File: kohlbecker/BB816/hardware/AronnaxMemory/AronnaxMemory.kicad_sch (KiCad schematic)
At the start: 29 parts, among them J1 Barrel_Jack_Switch, J2 Conn_02x40_Odd_Even, J3 Conn_02x18_Odd_Even, J5 I/O ~{CS}, J9 Vector Rewrite, U1 74LS04, U12 AS6C4008-55PCN, U13 AT28C256-15PC, U2 74LS32, U3 74LS32, U4 74LS08, U6 74LS32, U7 74LS32, U8 74LS138

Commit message: Cleanup
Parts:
- removed C6, C8: 100nF, Capacitor_THT:C_Disc_D3.4mm_W2.1mm_P2.50mm, symbol Device:C
- removed unit 4 of U2
- removed unit 5 of U2
- removed unit 2 of U2
- removed unit 1 of U2
- removed unit 1 of U6
- removed U7: 74LS32, Package_DIP:DIP-14_W7.62mm, symbol 74xx:74LS32
- removed U8: 74LS138, Package_DIP:DIP-16_W7.62mm, symbol 74xx:74LS138
- added C10, C11: 100nF, Capacitor_THT:C_Disc_D3.4mm_W2.1mm_P2.50mm, symbol Device:C
- added U10: 74HC30, Package_DIP:DIP-14_W7.62mm, symbol BB816:74HC30
- added U9: CD4072B, Package_DIP:DIP-14_W7.62mm, symbol cd4072B:4072
- renumbered U2 to U6
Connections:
- net A10: now also U10.2; no longer U6.5
- net A11: now also U10.3
- net A12: now also U10.4
- net A13: now also U10.5
- net A14: now also U10.6
- net A15: now also U1.1, U3.13; no longer U1.5, U3.10
- net A19: now also U1.9, U6.2; no longer U1.11, U6.10
- net A20: now also U9.5
- net A21: now also U9.4
- net A22: now also U9.3
- net A23: now also U9.2
- net A8: now also U10.11
- net A9: now also U10.12; no longer U6.4
- net E: now also U1.11, U4.13; no longer U1.1, U4.5
- net GND: now also J9.15 (Pin_15), J9.17 (Pin_17), J9.19 (Pin_19), J9.21 (Pin_21), U1.5, U4.4, U4.5, U6.10, U6.4, U6.5, U6.9, C10.2, C11.2, U10.7 (GND), U9.10, U9.11, U9.12, U9.7 (VSS), U9.9; no longer U1.9, U4.12, U4.13
- net VCC: now also C10.1, C11.1, U10.14 (VCC), U9.14 (VDD)
- net ~{BANK0_HI}: now also U1.13; no longer U1.3
- net ~{BANK0_LO}: now also U3.11, U10.1; no longer U3.8
- net ~{BANK0}: now also U3.12; no longer U3.9
- net ~{MEG0_LO}: now also U6.3; no longer U6.8
- net ~{PAGE1}: now also U1.4; no longer U1.13
- net ~{ROM_OE}: no longer U13.22 (~{OE})
- net at U3.4: now also U1.10; no longer U1.2
- net at U6.6: no longer U6.9
- net ~{A19}: now reaches U1.8
- net ~{A19}: now also U6.12
- net at U4.11: now also U3.9
- net ~{MEG0}: now reaches U6.13
- net ~{MEG0}: now also U6.1, U9.1; no longer U6.9
- net ~{MEG0_LO_OE}: now reaches U12.24 (OE#)
- net ~{MEG0_LO_OE}: now also U3.8; no longer U3.11
- net at U4.6: no longer U3.12
- net at U1.12: now also U4.12; no longer U3.13
- net at U1.6: no longer U3.1
- net ~{0x00}: no longer names the net of J5.20 (Pin_20)
- net ~{0x20}: no longer names the net of J5.18 (Pin_18)
- net ~{0x40}: no longer names the net of J5.16 (Pin_16)
- net ~{0x60}: no longer names the net of J5.14 (Pin_14)
- net ~{0x80}: no longer names the net of J5.12 (Pin_12)
- net ~{0xA0}: no longer names the net of J5.10 (Pin_10)
- net ~{0xCO}: no longer names the net of J5.8 (Pin_8)
- net ~{0xE0}: no longer names the net of J5.6 (Pin_6)
- new net PAGE1: U1.3, U10.8, U3.10
- new net ~{A15}: U1.2, U3.1
- no-connect marks 5 -> 8
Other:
- removed sheet VectorPullRewrite
- moved on the sheet: C1, C12, C13, C2, C3, C4, C5, C7, C9, D1, H1, H2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

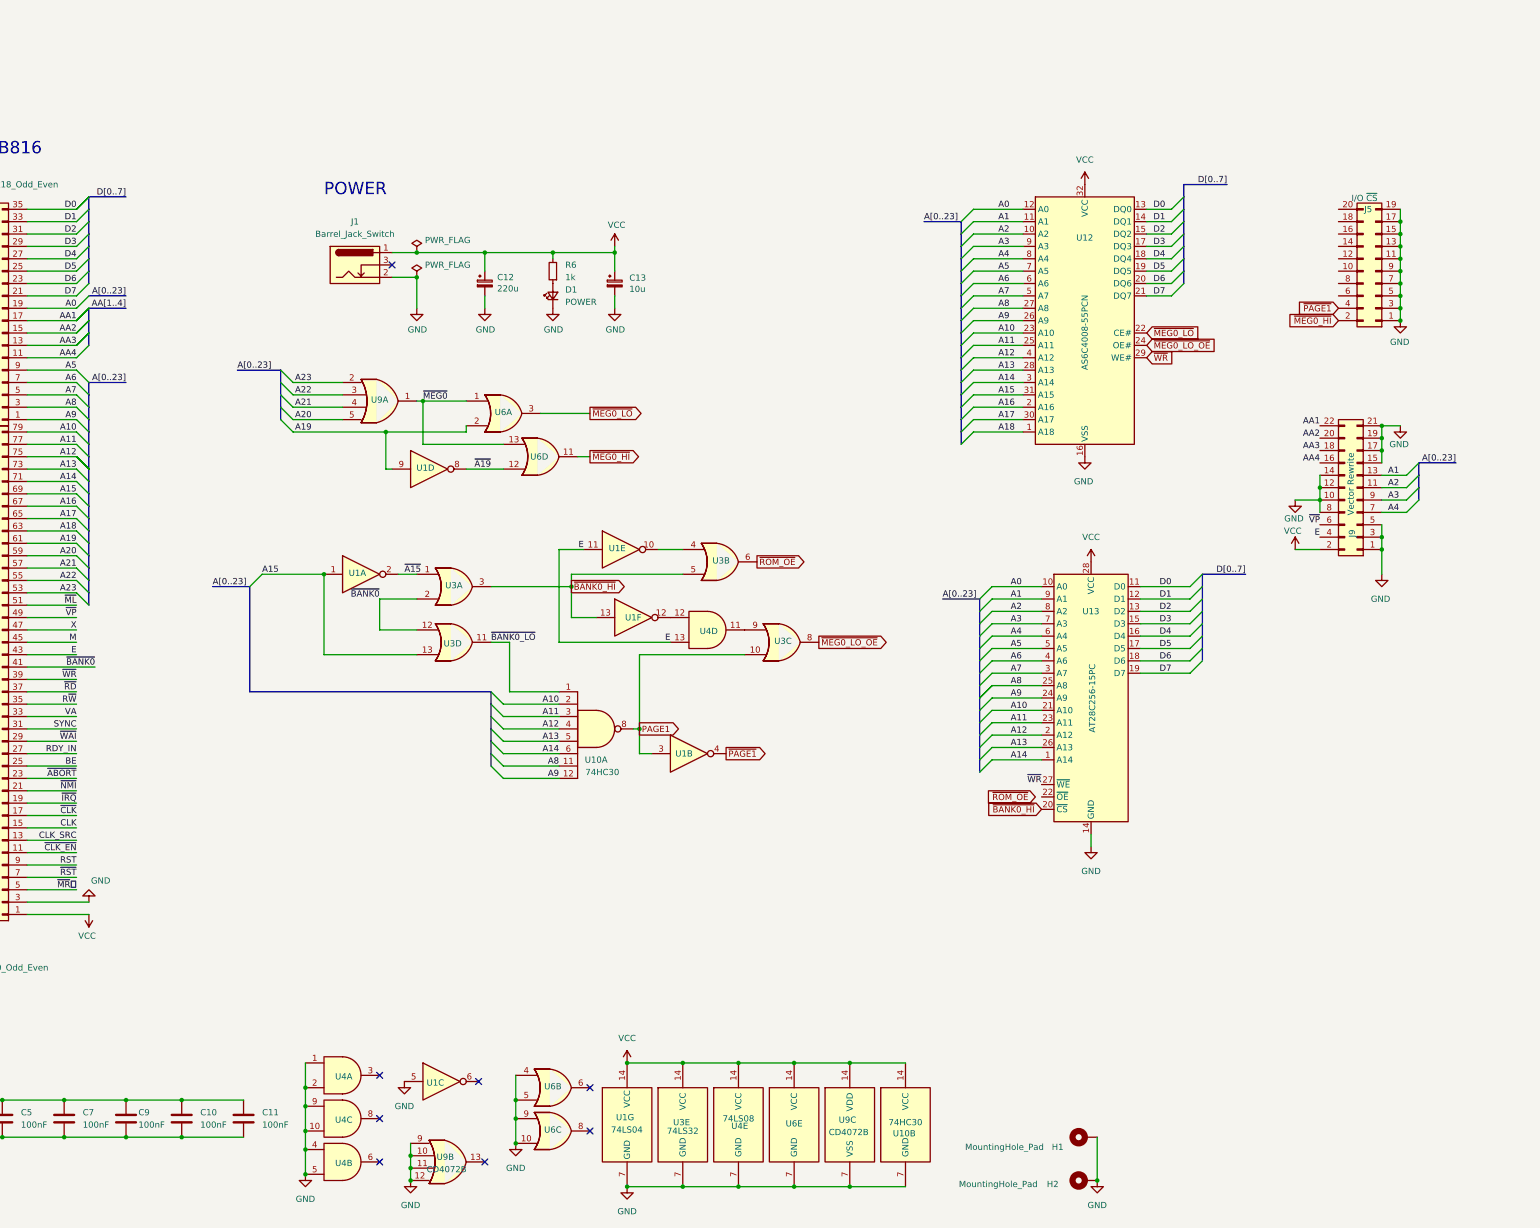
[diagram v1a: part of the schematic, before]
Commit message: ATF22V10
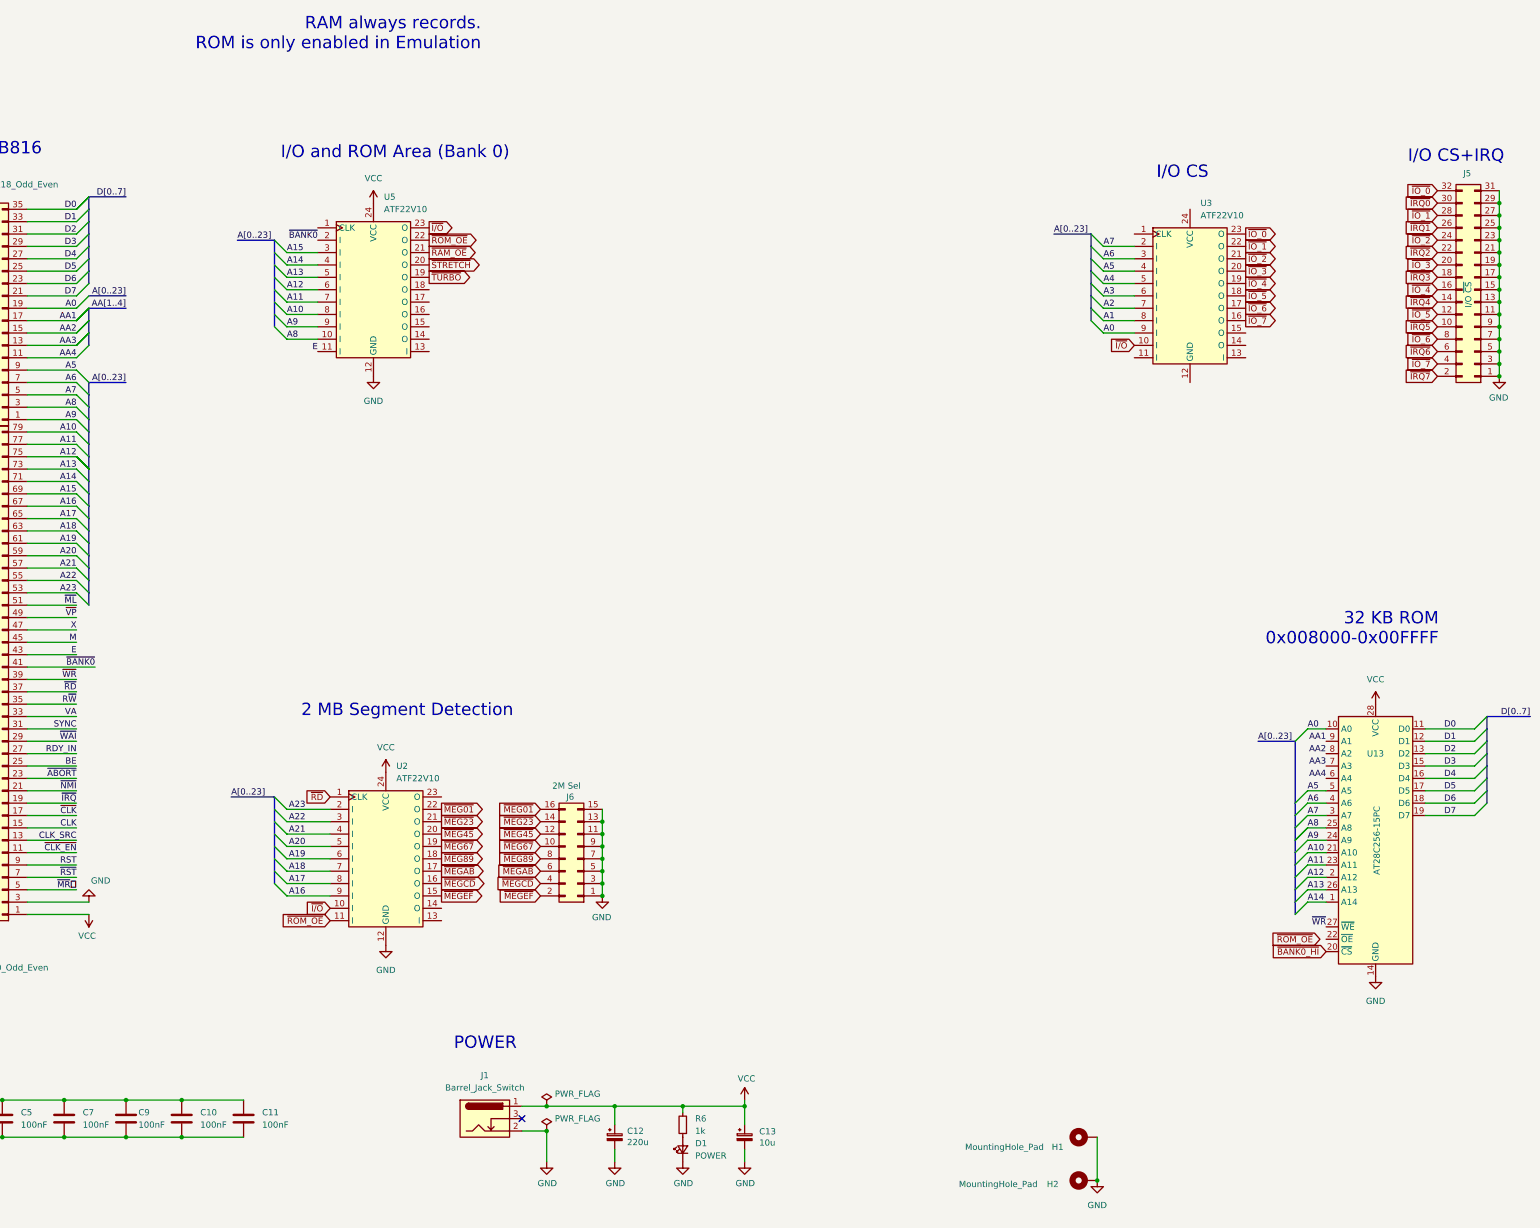
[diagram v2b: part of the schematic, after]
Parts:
- removed J9: Vector Rewrite, Connector_PinHeader_2.54mm:PinHeader_2x11_P2.54mm_Vertical, symbol Connector_Generic:Conn_02x11_Odd_Even
- removed U1: 74LS04, Package_DIP:DIP-14_W7.62mm, symbol 74xx:74LS04
- removed U10: 74HC30, Package_DIP:DIP-14_W7.62mm, symbol BB816:74HC30
- removed U12: AS6C4008-55PCN, Package_DIP:DIP-32_W15.24mm, symbol Memory_RAM:AS6C4008-55PCN
- removed U3, U6: 74LS32, Package_DIP:DIP-14_W7.62mm, symbol 74xx:74LS32
- removed U4: 74LS08, Package_DIP:DIP-14_W7.62mm, symbol 74xx:74LS08
- removed U9: CD4072B, Package_DIP:DIP-14_W7.62mm, symbol cd4072B:4072
- added J6: 2M Sel, Connector_PinHeader_2.54mm:PinHeader_2x10_P2.54mm_Vertical, symbol Connector_Generic:Conn_02x08_Odd_Even
- added U2, U3, U5: ATF22V10, Package_DIP:DIP-24_W7.62mm_Socket, symbol my:ATF22V10
- J5: symbol Connector_Generic:Conn_02x10_Odd_Even -> Connector_Generic:Conn_02x16_Odd_Even
- U13: footprint Socket:DIP_Socket-28_W11.9_W12.7_W15.24_W17.78_W18.5_3M_228-1277-00-0602J -> Package_DIP:DIP-28_W15.24mm_Socket
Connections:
- net A0: now also U3.9 (I)
- net A1: now also U3.8 (I); no longer U13.9 (A1)
- net A10: now also U5.8 (I)
- net A11: now also U5.7 (I)
- net A12: now also U5.6 (I)
- net A13: now also U5.5 (I)
- net A14: now also U5.4 (I)
- net A15: now also U5.3 (I)
- net A16: now also U2.9 (I)
- net A17: now also U2.8 (I)
- net A18: now also U2.7 (I)
- net A19: now also U2.6 (I)
- net A2: now also U3.7 (I); no longer U13.8 (A2)
- net A20: now also U2.5 (I)
- net A21: now also U2.4 (I)
- net A22: now also U2.3 (I)
- net A23: now also U2.2 (I)
- net A3: now also U3.6 (I); no longer U13.7 (A3)
- net A4: now also U3.5 (I); no longer U13.6 (A4)
- net A5: now also U3.4 (I)
- net A6: now also U3.3 (I)
- net A7: now also U3.2 (I)
- net A8: now also U5.10 (I)
- net A9: now also U5.9 (I)
- net AA1: now also U13.9 (A1)
- net AA2: now also U13.8 (A2)
- net AA3: now also U13.7 (A3)
- net AA4: now also U13.6 (A4)
- net E: now also U5.11 (I)
- net GND: now also J5.21 (Pin_21), J5.23 (Pin_23), J5.25 (Pin_25), J5.27 (Pin_27), J5.29 (Pin_29), J5.31 (Pin_31), J6.1 (Pin_1), J6.11 (Pin_11), J6.13 (Pin_13), J6.15 (Pin_15), J6.3 (Pin_3), J6.5 (Pin_5), J6.7 (Pin_7), J6.9 (Pin_9), U2.12 (GND), U5.12 (GND)
- net VCC: now also U2.24 (VCC), U5.24 (VCC)
- net ~{BANK0}: now also U5.2 (I)
- net ~{RD}: now also U2.1 (CLK)
- net ~{ROM_OE}: now also U2.11 (I), U5.22 (O)
- net ~{IRQ5}: now reaches J5.10 (Pin_10)
- net ~{IO_5}: now reaches J5.12 (Pin_12)
- net ~{IO_5}: now also U3.18 (O)
- net ~{IRQ4}: now reaches J5.14 (Pin_14)
- net ~{IO_4}: now reaches J5.16 (Pin_16)
- net ~{IO_4}: now also U3.19 (O)
- net ~{IRQ3}: now reaches J5.18 (Pin_18)
- net ~{IO_3}: now reaches J5.20 (Pin_20)
- net ~{IO_3}: now also U3.20 (O)
- net ~{IRQ6}: now reaches J5.6 (Pin_6)
- net ~{IO_6}: now reaches J5.8 (Pin_8)
- net ~{IO_6}: now also U3.17 (O)
- net ~{MEG0_HI} renamed ~{IRQ7}
- net ~{PAGE1} renamed ~{IO_7}
- net ~{IO_7}: now also U3.16 (O)
- new net ~{IO_0}: J5.32 (Pin_32), U3.23 (O)
- new net ~{IO_1}: J5.28 (Pin_28), U3.22 (O)
- new net ~{IO_2}: J5.24 (Pin_24), U3.21 (O)
- new net ~{IRQ0}: J5.30 (Pin_30)
- new net ~{IRQ1}: J5.26 (Pin_26)
- new net ~{IRQ2}: J5.22 (Pin_22)
- new net ~{I/O}: U2.10 (I), U3.10 (I), U5.23 (O)
- new net ~{MEG01}: J6.16 (Pin_16), U2.22 (O)
- new net ~{MEG23}: J6.14 (Pin_14), U2.21 (O)
- new net ~{MEG45}: J6.12 (Pin_12), U2.20 (O)
- new net ~{MEG67}: J6.10 (Pin_10), U2.19 (O)
- new net ~{MEG89}: J6.8 (Pin_8), U2.18 (O)
- new net ~{MEGAB}: J6.6 (Pin_6), U2.17 (O)
- new net ~{MEGCD}: J6.4 (Pin_4), U2.16 (O)
- new net ~{MEGEF}: J6.2 (Pin_2), U2.15 (O)
- new net ~{RAM_OE}: U5.21 (O)
- new net ~{STRETCH}: U5.20 (O)
- new net ~{TURBO}: U5.19 (O)
- no-connect marks 8 -> 1
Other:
- note added: "2 MB Segment Detection"
- note added: "32 KB ROM 0x008000-0x00FFFF"
- note added: "I/O CS"
- note added: "I/O CS+IRQ"
- note added: "I/O and ROM Area (Bank 0)"
- note added: "RAM always records. ROM is only enabled in Emulation"
- moved on the sheet: C12, C13, D1, J1, R6, U13

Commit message: PLAs for Days! Also Vector Rewrite
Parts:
- added D2, D3: 1N4148, Diode_THT:D_DO-35_SOD27_P7.62mm_Horizontal, symbol Diode:1N4148
- added J7: ~{IRQ7_NMI}, symbol Connector_Generic:Conn_02x02_Odd_Even
- added R1, R15: 1K, symbol Device:R
- added R13, R14, R3, R4, R5: 10K, symbol Device:R
- added RN1: 100k, Resistor_THT:R_Array_SIP9, symbol Device:R_Network08
- added U4: 74HC283, Package_DIP:DIP-16_W7.62mm_Socket, symbol Vega816:74HC283
- added U89: 74LS348, Package_DIP:DIP-16_W7.62mm_Socket, symbol 74xx:74LS348
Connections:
- net A1: now also U4.5 (A1)
- net A2: now also U4.3 (A2)
- net A3: now also U4.14 (A3)
- net A4: now also U4.12 (A4)
- net AA1: now also U4.10 (S4)
- net AA2: now also U4.13 (S3)
- net AA3: now also U4.1 (S2)
- net AA4: now also U4.4 (S1)
- net GND: now also R1.2, R15.2, R3.1, R4.1, R5.1, U4.11 (B4), U4.7 (C0), U4.8 (GND), U89.8 (GND)
- net VCC: now also D3.1 (K), J7.1 (Pin_1), R13.1, R14.1, U4.16 (VCC), U89.16 (VCC)
- net ~{IRQ0}: now also RN1.2 (R1), U89.4 (7)
- net ~{IRQ1}: now also RN1.3 (R2), U89.3 (6)
- net ~{IRQ2}: now also RN1.4 (R3), U89.2 (5)
- net ~{IRQ3}: now also RN1.5 (R4), U89.1 (4)
- net ~{IRQ4}: now also RN1.6 (R5), U89.13 (3)
- net ~{IRQ5}: now also RN1.7 (R6), U89.12 (2)
- net ~{IRQ6}: now also RN1.8 (R7), U89.11 (1)
- net ~{IRQ7}: now also J7.2 (Pin_2), J7.4 (Pin_4), RN1.9 (R8)
- net ~{IRQ}: now also D3.2 (A)
- net ~{NMI}: now also D2.2 (A)
- net ~{VP}: now also U3.11 (I)
- net ~{VP_REWRITE}: now reaches U3.14 (O)
- net ~{VP_REWRITE}: now also U89.5 (EI)
- new net: J7.3 (Pin_3), U89.10 (0)
- new net: R14.2, U89.14 (GS)
- new net: D2.1 (K), R13.2
- new net Y1: R5.2, U4.6 (B1), U89.9 (A0)
- new net Y2: R4.2, U4.2 (B2), U89.7 (A1)
- new net Y3: R3.2, U4.15 (B3), U89.6 (A2)
- no-connect marks 1 -> 3
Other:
- note added: "IRQ Priority"
- note added: "Reversed? Swap pins in symbol?"
- note added: "Vector Address Rewrite"
- note added: "~{VPB}+~{IRQ} Rewrite"
- note removed: "RAM always records. ROM is only enabled in Emulation"
- moved on the sheet: J2, J3, J5, J6, U13, U2, U3, U5
